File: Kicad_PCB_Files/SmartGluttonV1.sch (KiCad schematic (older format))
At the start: 27 parts, among them J1 mDot breakout, J2 FLOW CONTROL, J3 mDot pin11-20 brkout, J4 mDot pin1-10 brkout, J5 USB_A, J6 USB_B, J7 GPS Connector, J8 Ultrasonic Conn, SW1 UART_PWR, SW2 Reset, U1 FT231XS, U2 MCP1700-3002E_TO92

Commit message: Add files via upload
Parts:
- C1, C2, C3, C4, C5, C6, J5, R1, R10, R2, R9, SW1, U2: Vendor (none) -> ETSG
- FB1: Vendor (none) -> rs-online https://au.rs-online.com/web/p/wire-wound-surface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
- J6: Vendor (none) -> https://au.rs-online.com/web/p/type-b-usb-connectors/800686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
- J8: footprint (none) -> Connector_PinSocket_2.54mm:PinSocket_1x04_P2.54mm_Vertical
- MCU1: Vendor (none) -> 2mm pitch headers 10x1 10x1 8x1
- SW2: Vendor (none) -> ETSG 6x6x4.3
- U1: Vendor (none) -> https://au.rs-online.com/web/p/universal-asynchronous-recei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
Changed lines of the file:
@@
 F 2 "Package_TO_SOT_THT:TO-92_HandSolder" H 6200 1350 50  0001 C CIN
 F 3 "http://ww1.microchip.com/downloads/en/DeviceDoc/20001826D.pdf" H 6200 1550 50  0001 C CNN
+F 4 "ETSG" H 6200 1550 50  0001 C CNN "Vendor"
 	1    6200 1550
 	-1   0    0    1
@@
 F 2 "SmartGluttonV1:USB_B_Molex_USB-67068-xx1x_StraightTab_Horizontal" H 10150 1450 50  0001 C CNN
 F 3 " ~" H 10150 1450 50  0001 C CNN
+F 4 "https://au.rs-online.com/web/p/type-b-usb-connectors/8006860/" H 10000 1500 50  0001 C CNN "Vendor"
 	1    10000 1500
 	-1   0    0    -1
@@
 F 2 "Package_SO:SSOP-20_3.9x8.7mm_P0.635mm" H 4150 3900 50  0001 C CNN
 F 3 "http://www.ftdichip.com/Products/ICs/FT231X.html" H 3550 4850 50  0001 C CNN
+F 4 "https://au.rs-online.com/web/p/universal-asynchronous-receivers-transmitters/7570032/" H 3550 4850 50  0001 C CNN "Vendor"
 	1    3550 4850
 	1    0    0    -1
@@
 F 2 "Resistor_SMD:R_0805_2012Metric_Pad1.15x1.40mm_HandSolder" V 2230 4550 50  0001 C CNN
 F 3 "~" H 2300 4550 50  0001 C CNN
+F 4 "ETSG" V 2300 4550 50  0001 C CNN "Vendor"
 	1    2300 4550
 	0    1    1    0
@@
 F 2 "Resistor_SMD:R_0805_2012Metric_Pad1.15x1.40mm_HandSolder" V 2230 4650 50  0001 C CNN
 F 3 "~" H 2300 4650 50  0001 C CNN
+F 4 "ETSG" V 2300 4650 50  0001 C CNN "Vendor"
 	1    2300 4650
 	0    1    1    0
@@
 F 2 "Capacitor_SMD:C_0805_2012Metric_Pad1.15x1.40mm_HandSolder" H 1738 4650 50  0001 C CNN
 F 3 "~" H 1700 4800 50  0001 C CNN
+F 4 "ETSG" H 1700 4800 50  0001 C CNN "Vendor"
 	1    1700 4800
 	1    0    0    -1
@@
 F 2 "Capacitor_SMD:C_0805_2012Metric_Pad1.15x1.40mm_HandSolder" H 1288 4650 50  0001 C CNN
 F 3 "~" H 1250 4800 50  0001 C CNN
+F 4 "ETSG" H 1250 4800 50  0001 C CNN "Vendor"
 	1    1250 4800
 	1    0    0    -1
@@
 F 2 "Capacitor_SMD:C_0805_2012Metric_Pad1.15x1.40mm_HandSolder" H 2488 3950 50  0001 C CNN
 F 3 "~" H 2450 4100 50  0001 C CNN
+F 4 "ETSG" H 2450 4100 50  0001 C CNN "Vendor"
 	1    2450 4100
 	1    0    0    -1
@@
 F 2 "Capacitor_SMD:C_0805_2012Metric_Pad1.15x1.40mm_HandSolder" H 1238 1100 50  0001 C CNN
 F 3 "~" H 1200 1250 50  0001 C CNN
+F 4 "ETSG" H 1200 1250 50  0001 C CNN "Vendor"
 	1    1200 1250
 	1    0    0    -1
@@
 F 2 "SmartGluttonV1:mdot" H 7050 5050 50  0001 C CNN
 F 3 "" H 7050 5050 50  0001 C CNN
+F 4 "2mm pitch headers 10x1 10x1 8x1" V 7050 5050 50  0001 C CNN "Vendor"
 	1    7050 5050
 	0    1    1    0
@@
 F 2 "Inductor_SMD:L_0603_1608Metric_Pad1.05x0.95mm_HandSolder" V 5330 3250 50  0001 C CNN
 F 3 "~" H 5400 3250 50  0001 C CNN
+F 4 "rs-online https://au.rs-online.com/web/p/wire-wound-surface-mount-inductors/7242989/" V 5400 3250 50  0001 C CNN "Vendor"
 	1    5400 3250
 	0    1    1    0
@@
 F 2 "Capacitor_THT:CP_Radial_D5.0mm_P2.50mm" H 5138 3250 50  0001 C CNN
 F 3 "~" H 5100 3400 50  0001 C CNN
+F 4 "ETSG" H 5100 3400 50  0001 C CNN "Vendor"
 	1    5100 3400
 	1    0    0    -1
@@
 F 2 "Capacitor_SMD:C_0805_2012Metric_Pad1.15x1.40mm_HandSolder" H 4788 3250 50  0001 C CNN
 F 3 "~" H 4750 3400 50  0001 C CNN
+F 4 "ETSG" H 4750 3400 50  0001 C CNN "Vendor"
 	1    4750 3400
 	1    0    0    -1
@@
 F 2 "SmartGluttonV1:USB_A_FCI_87583_Horizontal" H 9750 5000 50  0001 C CNN
 F 3 " ~" H 9750 5000 50  0001 C CNN
+F 4 "ETSG" H 9600 5050 50  0001 C CNN "Vendor"
 	1    9600 5050
 	-1   0    0    -1
@@
 F 2 "Button_Switch_THT:SW_PUSH_6mm" H 750 1700 50  0001 C CNN
 F 3 "~" H 750 1700 50  0001 C CNN
+F 4 "ETSG 6x6x4.3" V 750 1500 50  0001 C CNN "Vendor"
 	1    750  1500
 	0    1    1    0
@@
 F 2 "Resistor_SMD:R_0805_2012Metric_Pad1.15x1.40mm_HandSolder" V 10030 2150 50  0001 C CNN
 F 3 "~" H 10100 2150 50  0001 C CNN
+F 4 "ETSG" H 10100 2150 50  0001 C CNN "Vendor"
 	1    10100 2150
 	1    0    0    -1
@@
 F 2 "Resistor_SMD:R_0805_2012Metric_Pad1.15x1.40mm_HandSolder" V 9630 5600 50  0001 C CNN
 F 3 "~" H 9700 5600 50  0001 C CNN
+F 4 "ETSG" H 9700 5600 50  0001 C CNN "Vendor"
 	1    9700 5600
 	1    0    0    -1
@@
 F 0 "J8" V 7488 1862 50  0000 R CNN
 F 1 "Ultrasonic Conn" V 7397 1862 50  0000 R CNN
-F 2 "" H 7550 2150 50  0001 C CNN
+F 2 "Connector_PinSocket_2.54mm:PinSocket_1x04_P2.54mm_Vertical" H 7550 2150 50  0001 C CNN
 F 3 "~" H 7550 2150 50  0001 C CNN
 	1    7550 2150
@@
 F 2 "Package_DIP:DIP-4_W7.62mm_LongPads" H 4000 3350 50  0001 C CNN
 F 3 "~" H 4000 3350 50  0001 C CNN
+F 4 "ETSG" H 4000 3350 50  0001 C CNN "Vendor"
 	1    4000 3350
 	-1   0    0    -1

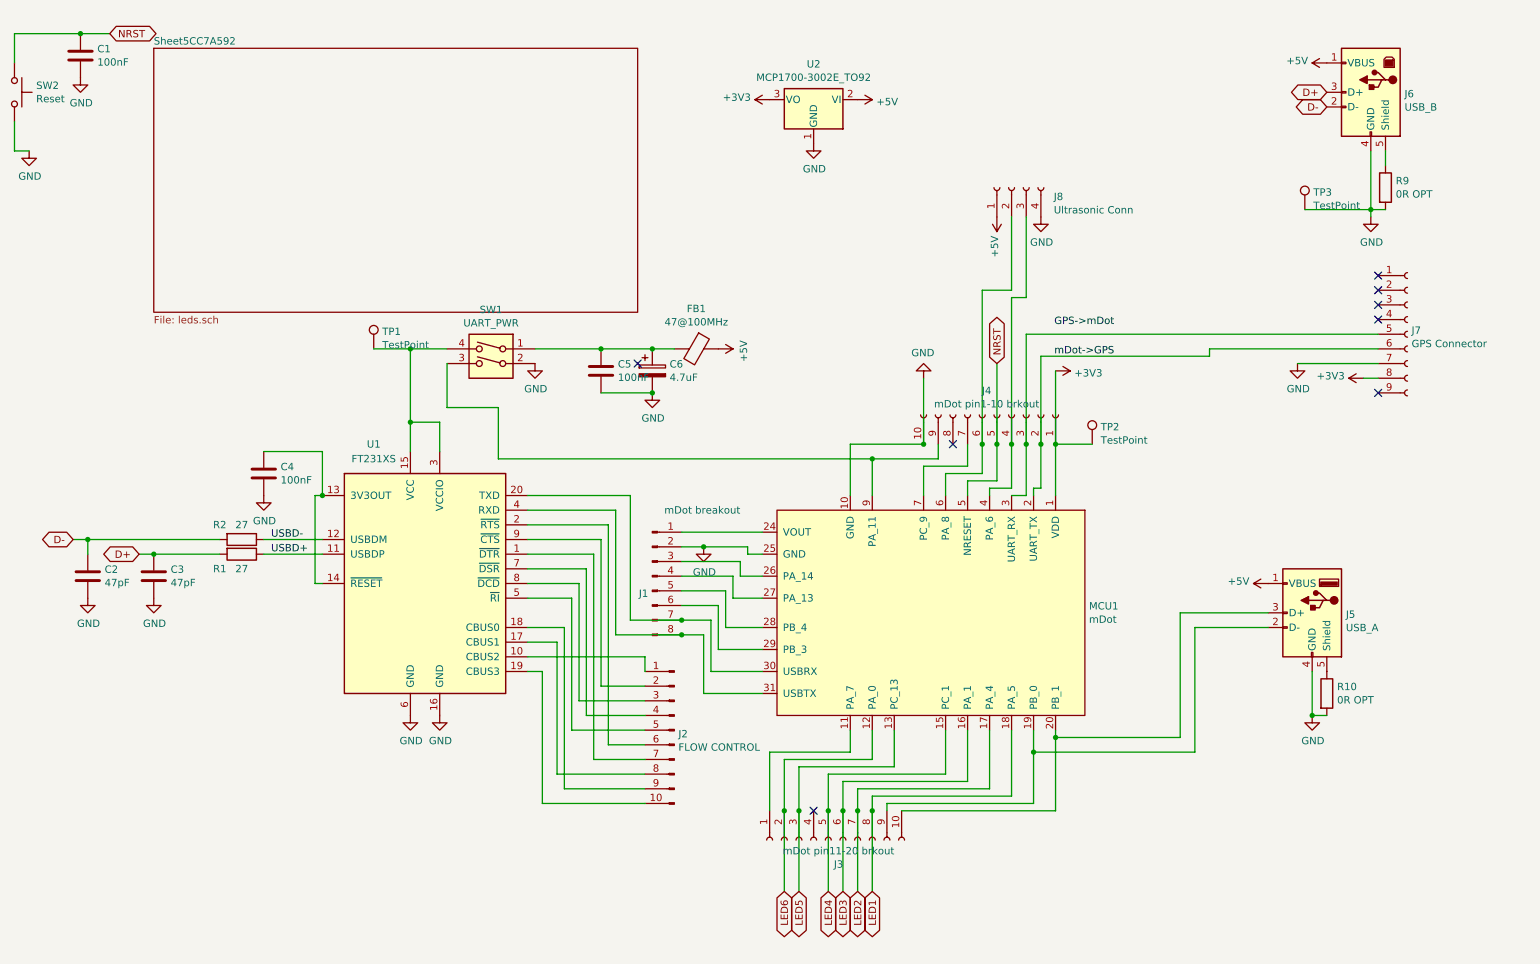
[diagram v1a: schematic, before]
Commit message: Add files via upload
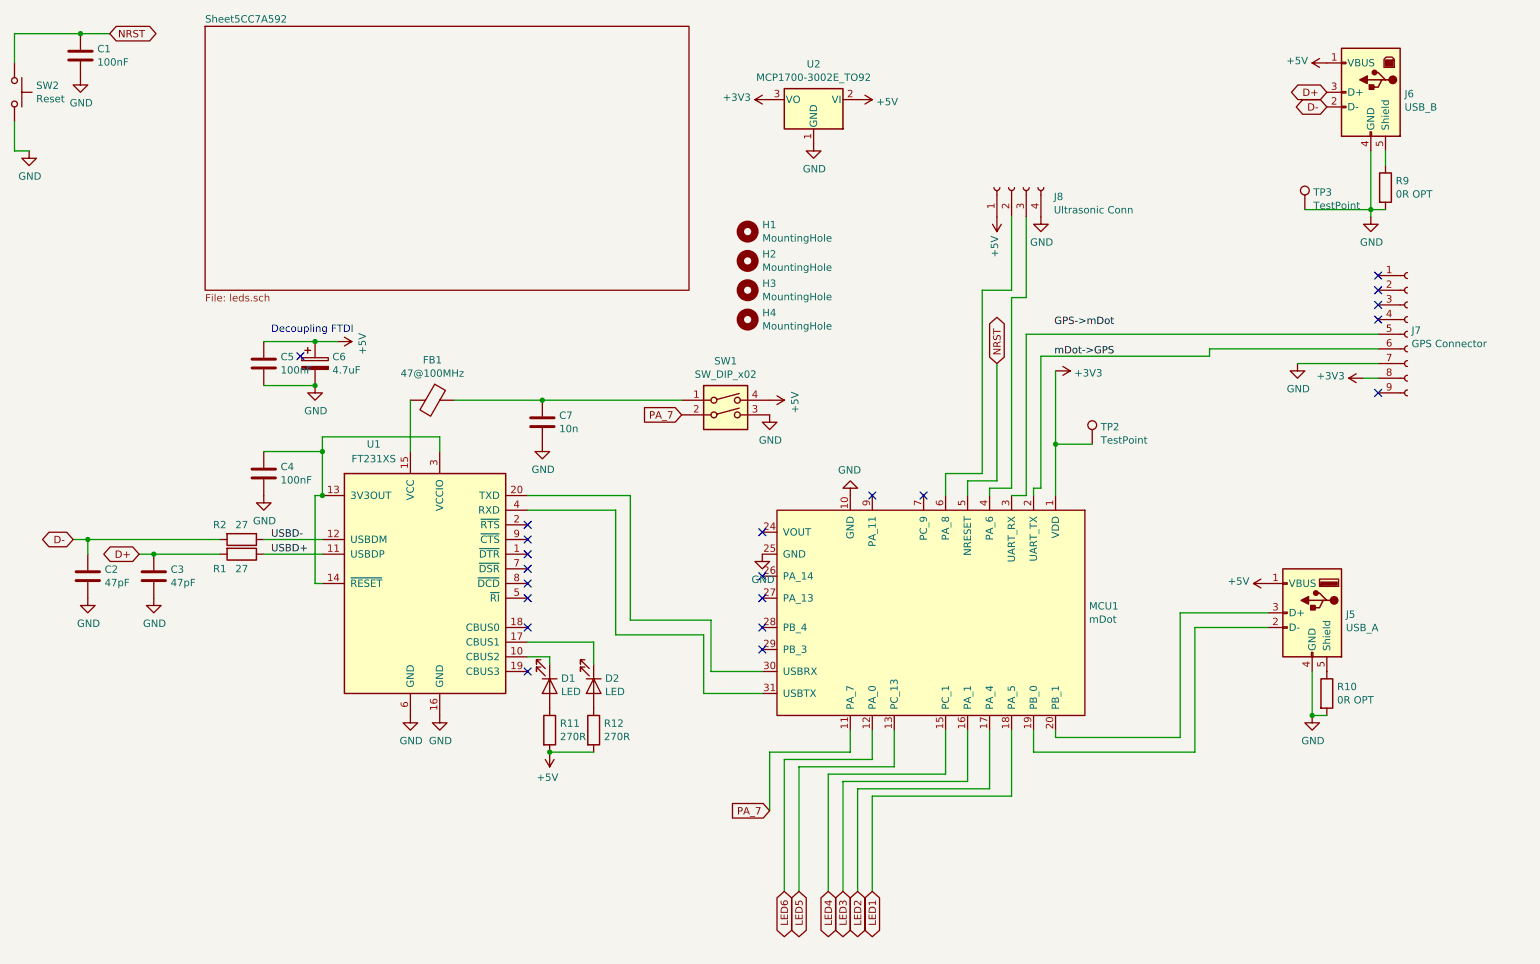
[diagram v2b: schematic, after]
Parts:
- removed J1: mDot breakout, Connector_PinHeader_2.54mm:PinHeader_1x08_P2.54mm_Vertical, symbol Connector:Conn_01x08_Male
- removed J2: FLOW CONTROL, Connector_PinHeader_2.54mm:PinHeader_1x10_P2.54mm_Vertical, symbol Connector:Conn_01x10_Male
- removed J3: mDot pin11-20 brkout, Connector_PinHeader_2.54mm:PinHeader_1x10_P2.54mm_Vertical, symbol Connector:Conn_01x10_Female
- removed J4: mDot pin1-10 brkout, Connector_PinHeader_2.54mm:PinHeader_1x10_P2.54mm_Vertical, symbol Connector:Conn_01x10_Female
- removed TP1: TestPoint, TestPoint:TestPoint_Pad_3.0x3.0mm, symbol Connector:TestPoint
- added C7: 10n, Capacitor_SMD:C_0805_2012Metric_Pad1.15x1.40mm_HandSolder, symbol Device:C
- added D1, D2: LED, LED_SMD:LED_0805_2012Metric_Pad1.15x1.40mm_HandSolder, symbol Device:LED
- added H1, H2, H3, H4: MountingHole, MountingHole:MountingHole_4mm, symbol Mechanical:MountingHole
- added R11, R12: 270R, Resistor_SMD:R_0805_2012Metric_Pad1.15x1.40mm_HandSolder, symbol Device:R
- SW1: value UART_PWR -> SW_DIP_x02; footprint Package_DIP:DIP-4_W7.62mm_LongPads -> Package_DIP:DIP-4_W8.89mm_SMDSocket_LongPads
- U1: footprint Package_SO:SSOP-20_3.9x8.7mm_P0.635mm -> SmartGluttonV1:SSOP-20_3.9x8.7mm_P0.635mm_HandSolder
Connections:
- net +5V: now also C5.1, C6.1, SW1.4, R11.2, R12.2; no longer FB1.1
- net GND: now also SW1.3, C7.2; no longer SW1.2
- net at U1.10 (CBUS2): now also D1.1 (K)
- net at C4.1, U1.13 (3V3OUT), U1.14 (~RESET): now also U1.3 (VCCIO)
- net at U1.17 (CBUS1): now also D2.1 (K)
- net PA_7: now reaches MCU1.11 (PA_7)
- net PA_7: now also SW1.2
- net at MCU1.9 (PA_11): no longer SW1.3
- new net: FB1.2, U1.15 (VCC)
- new net: C7.1, FB1.1, SW1.1
- new net: D2.2 (A), R12.1
- new net: D1.2 (A), R11.1
- no-connect marks 8 -> 21
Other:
- note added: "Decoupling FTDI"
- moved on the sheet: C5, C6, FB1

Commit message: Add files via upload
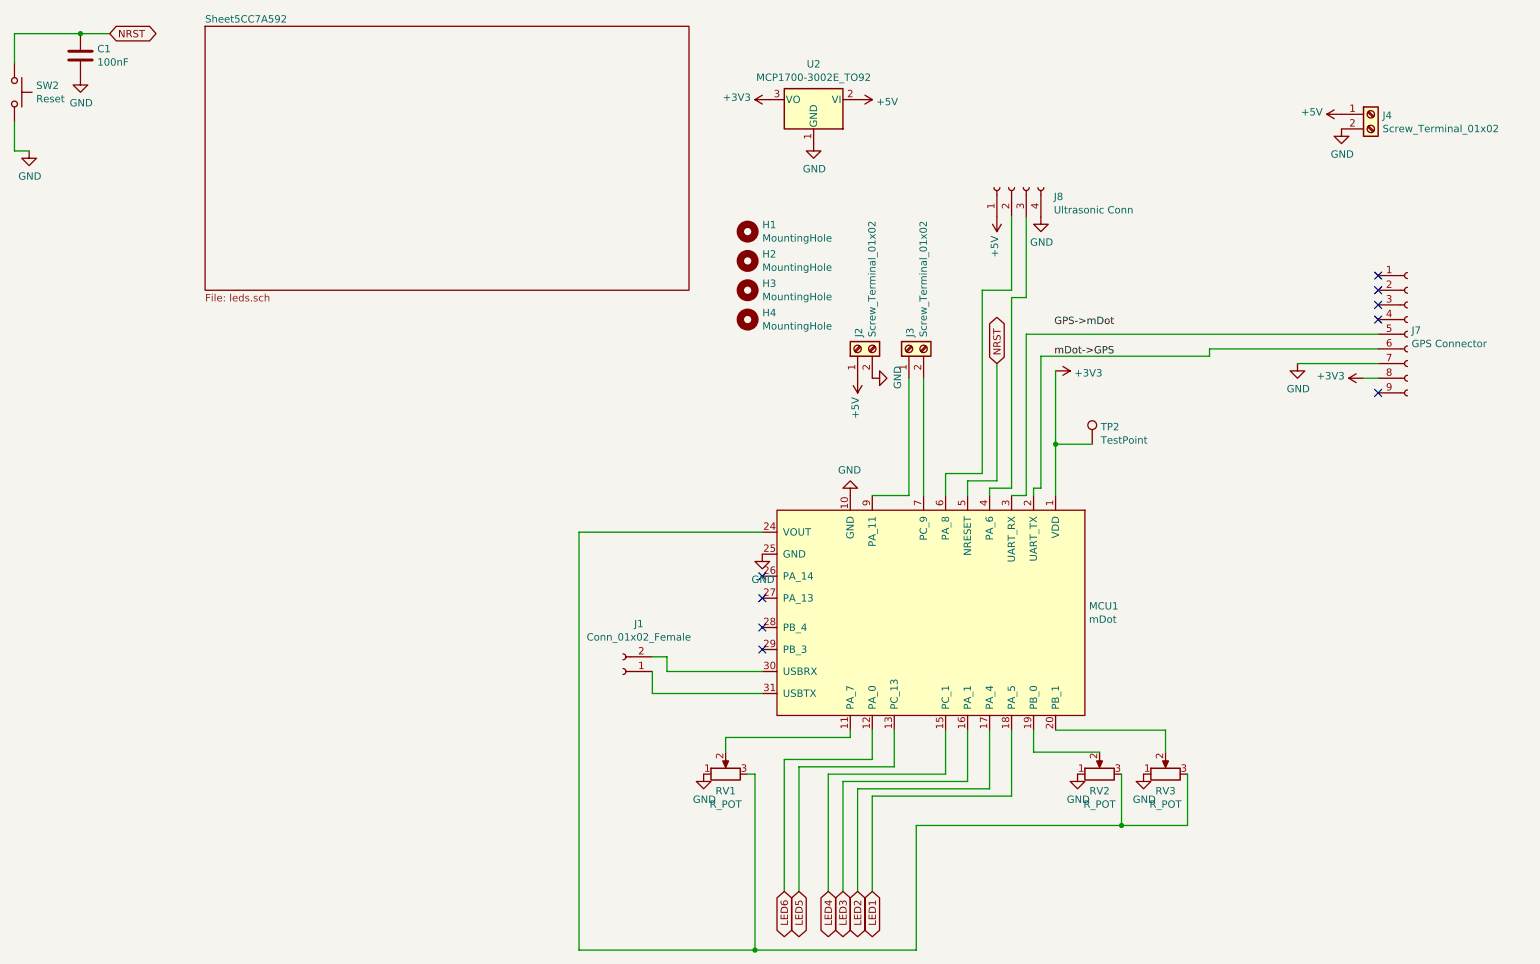
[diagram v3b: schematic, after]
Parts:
- removed C2, C3: 47pF, Capacitor_SMD:C_0805_2012Metric_Pad1.15x1.40mm_HandSolder, symbol Device:C
- removed C4, C5: 100nF, Capacitor_SMD:C_0805_2012Metric_Pad1.15x1.40mm_HandSolder, symbol Device:C
- removed C6: 4.7uF, Capacitor_THT:CP_Radial_D5.0mm_P2.50mm, symbol Device:CP
- removed C7: 10n, Capacitor_SMD:C_0805_2012Metric_Pad1.15x1.40mm_HandSolder, symbol Device:C
- removed D1, D2: LED, LED_SMD:LED_0805_2012Metric_Pad1.15x1.40mm_HandSolder, symbol Device:LED
- removed FB1: 47@100MHz, Inductor_SMD:L_0603_1608Metric_Pad1.05x0.95mm_HandSolder, symbol Device:Ferrite_Bead
- removed J5: USB_A, SmartGluttonV1:USB_A_FCI_87583_Horizontal, symbol Connector:USB_A
- removed J6: USB_B, SmartGluttonV1:USB_B_Molex_USB-67068-xx1x_StraightTab_Horizontal, symbol Connector:USB_B
- removed R1, R2: 27, Resistor_SMD:R_0805_2012Metric_Pad1.15x1.40mm_HandSolder, symbol Device:R
- removed R10, R9: 0R OPT, Resistor_SMD:R_0805_2012Metric_Pad1.15x1.40mm_HandSolder, symbol Device:R
- removed R11, R12: 270R, Resistor_SMD:R_0805_2012Metric_Pad1.15x1.40mm_HandSolder, symbol Device:R
- removed SW1: SW_DIP_x02, Package_DIP:DIP-4_W8.89mm_SMDSocket_LongPads, symbol Switch:SW_DIP_x02
- removed TP3: TestPoint, TestPoint:TestPoint_Pad_3.0x3.0mm, symbol Connector:TestPoint
- removed U1: FT231XS, SmartGluttonV1:SSOP-20_3.9x8.7mm_P0.635mm_HandSolder, symbol Interface_USB:FT231XS
- added J1: Conn_01x02_Female, Connector_PinHeader_2.54mm:PinHeader_1x02_P2.54mm_Vertical, symbol Connector:Conn_01x02_Female
- added J2, J3, J4: Screw_Terminal_01x02, TerminalBlock:TerminalBlock_bornier-2_P5.08mm, symbol Connector:Screw_Terminal_01x02
- added RV1, RV2, RV3: R_POT, Potentiometer_THT:Potentiometer_Bourns_3296W_Vertical, symbol Device:R_POT
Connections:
- net +5V: now also J2.1 (Pin_1), J4.1 (Pin_1)
- net GND: now also J2.2 (Pin_2), J4.2 (Pin_2), RV1.1, RV2.1, RV3.1
- net at MCU1.30 (USBRX): now also J1.2 (Pin_2)
- net at MCU1.31 (USBTX): now also J1.1 (Pin_1)
- net at MCU1.19 (PB_0): now also RV2.2
- net at MCU1.20 (PB_1): now also RV3.2
- net at MCU1.24 (VOUT): now also RV1.3, RV2.3, RV3.3
- net at MCU1.7 (PC_9): now also J3.2 (Pin_2)
- net at MCU1.9 (PA_11): now also J3.1 (Pin_1)
- net PA_7: no longer names the net of MCU1.11 (PA_7)
- net PA_7: now also RV1.2
- no-connect marks 21 -> 9
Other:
- note removed: "Decoupling FTDI"
